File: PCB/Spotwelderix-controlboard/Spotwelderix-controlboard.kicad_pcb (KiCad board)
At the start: 2 copper layers, 65.6 x 60 mm, 35 parts, among them J1 ChargerPower, J2 LEDs, J3 ExtPwr_FAn, P1 Display, P2 PowerPCB, Q1 AO3400A, Q2 AO3400A, Q5 AO3400A, U1 NodeMCU32, U3 LM7805M_TO263

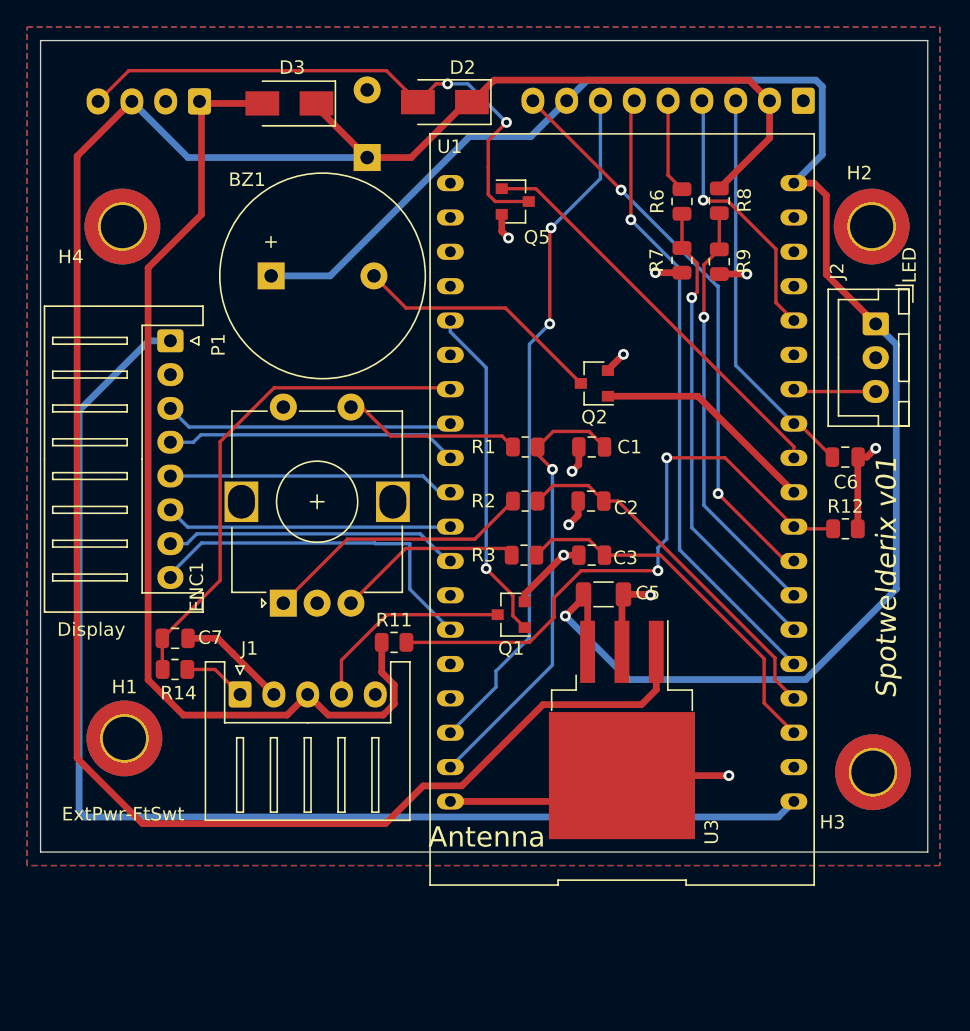
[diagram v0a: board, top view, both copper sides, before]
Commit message: V2 tweaks and tricks
Voltmeasure enable
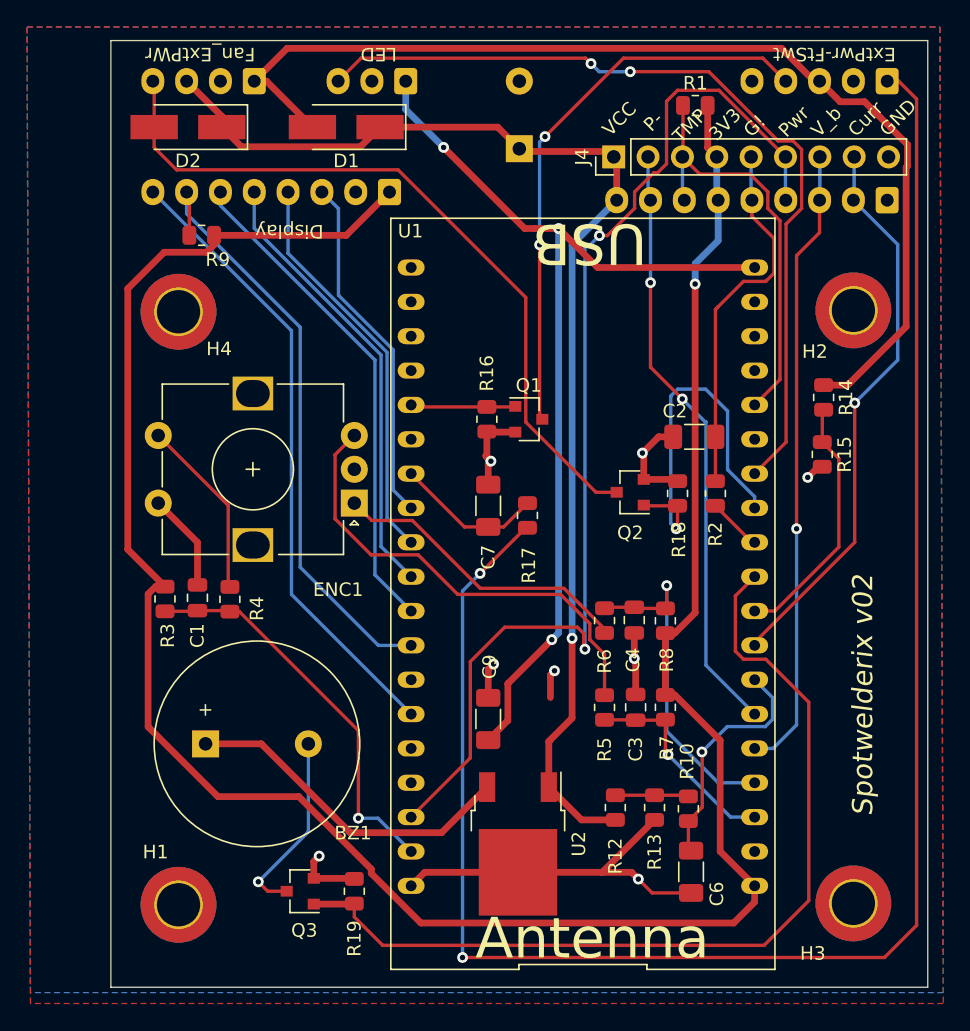
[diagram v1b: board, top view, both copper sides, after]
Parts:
- removed the R6 at (67.4, 31.9)
- added C6: 470p, Capacitor_SMD:C_1206_3216Metric_Pad1.33x1.80mm_HandSolder, F.Cu at (68.1, 81.5)
- added J4: Testpin, Connector_PinHeader_2.54mm:PinHeader_1x09_P2.54mm_Vertical, F.Cu at (62.4, 28.6)
- added R1: 2.5k, Resistor_SMD:R_0805_2012Metric, F.Cu at (68.4, 24.8)
- added R10: 47k, Resistor_SMD:R_0805_2012Metric, F.Cu at (67.9, 76.8)
- added R16: 10k, Resistor_SMD:R_0805_2012Metric, F.Cu at (53.0, 48.0)
- added R18: 10k, Resistor_SMD:R_0805_2012Metric, F.Cu at (67.1, 53.5)
- added R19: 10k, Resistor_SMD:R_0805_2012Metric, F.Cu at (43.2, 82.9)
- added R2: 100, Resistor_SMD:R_0805_2012Metric, F.Cu at (69.9, 53.5)
- added R3: 2.5k, Resistor_SMD:R_0805_2012Metric, F.Cu at (29.2, 61.3)
- added R8: 2.5k, Resistor_SMD:R_0805_2012Metric, F.Cu at (66.2, 62.9)
- added R9: 2.5k, Resistor_SMD:R_0805_2012Metric, F.Cu at (31.9, 34.4)
- C2: renamed from C6; footprint Capacitor_SMD:C_0805_2012Metric -> Capacitor_SMD:C_1206_3216Metric_Pad1.33x1.80mm_HandSolder
- C7: footprint Capacitor_SMD:C_0805_2012Metric -> Capacitor_SMD:C_1206_3216Metric_Pad1.33x1.80mm_HandSolder
- C9: renamed from C5; footprint Capacitor_SMD:C_1206_3216Metric -> Capacitor_SMD:C_1206_3216Metric_Pad1.33x1.80mm_HandSolder
- D1: renamed from D3; footprint Diode_SMD:D_SMA -> Diode_SMD:D_SMA_Handsoldering
- D2: footprint Diode_SMD:D_SMA -> Diode_SMD:D_SMA_Handsoldering
- J1: renamed from J2; moved to B.Cu
- J2: renamed from J1; footprint Connector_JST:JST_XH_S5B-XH-A_1x05_P2.50mm_Horizontal -> Connector_JST:JST_XH_B5B-XH-A_1x05_P2.50mm_Vertical; moved to B.Cu
- P1: footprint Connector_JST:JST_XH_S8B-XH-A_1x08_P2.50mm_Horizontal -> Connector_JST:JST_XH_B8B-XH-A_1x08_P2.50mm_Vertical; moved to B.Cu
- P2: value PowerPCB -> CONN_01X08
- R12: renamed from R8; value 33k -> 15k
- R13: renamed from R9; value 10k -> 2.5k
- R14: renamed from R11; value 33k -> 15k
- R15: renamed from R12; value 10k -> 2.5k
- R7: value 10k -> 2.5k
- U2: renamed from U3; footprint Package_TO_SOT_SMD:TO-263-3_TabPin2 -> Package_TO_SOT_SMD:TO-252-2
- moved J2 65.9 mm to (82.6, 23.0), turned to 180 degrees
- moved R12 45.5 mm to (62.5, 76.7), turned to 90 degrees
- moved Q3 43.4 mm to (39.2, 82.9)
- moved R13 40.6 mm to (65.4, 76.7)
- moved J1 39.1 mm to (47.0, 23.0), turned to 180 degrees
- moved R14 36.6 mm to (77.9, 46.4), turned to 270 degrees
- moved BZ1 34.9 mm to (32.2, 72.0)
- moved R7 33.1 mm to (66.2, 69.3), turned to 90 degrees
- moved C1 31.2 mm to (31.6, 61.2), turned to 90 degrees
- moved R17 28.4 mm to (56.0, 55.1), turned to 270 degrees
- moved C7 25.1 mm to (53.1, 54.4), turned to 90 degrees
- moved R4 24.6 mm to (34.0, 61.3), turned to 90 degrees
- moved Q2 23.1 mm to (63.6, 53.4), turned to 180 degrees
- moved P1 19.6 mm to (45.8, 31.2), turned to 180 degrees
- moved D2 19.1 mm to (30.9, 26.4)
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- renumbered C2 to C4, C4 to C8, Q5 to Q2, Q2 to Q3, R14 to R17, R1 to R4, R3 to R5, R2 to R6
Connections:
- P2 pad 2: VCC -> Shuntvoltage
- P2 pad 3: Gate_logic -> Vbat_ADC
- P2 pad 4: Dallas -> EnableSupply
- P2 pad 5: Probe -> Gate_logic
- P2 pad 6: Vbat_ADC -> +3V3
- P2 pad 7: EnableSupply -> Dallas
- P2 pad 8: +5V -> ProbeADC
- P2 pad 9: Shuntvoltage -> VCC
- R12 pad 2: VCC_ADC -> Net-(R10-Pad2)
- R13 pad 1: VCC_ADC -> Net-(R10-Pad2)
- R7 pad 1: ProbeADC -> UI_RotEnc_B
- R7 pad 2: GND -> +3V3
- U1 pad 11: FAN -> Net-(R2-Pad2)
- U1 pad 12: Gate_logic -> FAN
- U1 pad 18: GND -> Net-(U1-Pad18)
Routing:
- net Net-(J2-Pad1): track 5.30 -> 132.2 mm, vias 0 -> 2
- net +3V3: track 92.0 -> 173.3 mm, vias 0 -> 1
- net VCC: track 167.8 -> 90.4 mm, vias 0 -> 1
- net LED: track 6.12 -> 63.2 mm, vias 0 -> 2
- net BUZZ: track 16.7 -> 67.6 mm
- net EnableSupply: track 51.3 -> 82.2 mm
- net +5V: track 124.7 -> 97.7 mm, vias 1 -> 3
- net Net-(J2-Pad4): track 15.5 -> 42.1 mm, vias 0 -> 2
- net FootSwitch: track 37.4 -> 11.0 mm
- net ExtPWRADC: track 44.7 -> 18.9 mm, vias 2 -> 0
- net Net-(P1-Pad7): track 21.8 -> 45.1 mm
- net Net-(ENC1-PadB): track 13.8 -> 34.5 mm
- net Net-(P1-Pad8): track 26.5 -> 46.5 mm
- net ChargerEna: track 25.0 -> 7.78 mm, vias 1 -> 0
- net Net-(P1-Pad6): track 21.2 -> 36.8 mm
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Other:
- board size 65.6 x 60 mm -> 60.4 x 70 mm
- board text added: "3V3"
- board text added: "Curr"
- board text added: "Fan_ExtPWr"
- board text added: "G!"
- board text added: "GND"
- board text added: "P-"
- board text added: "Pwr"
- board text added: "Spotwelderix v02"
- board text added: "TMP"
- board text added: "USB"
- board text added: "VCC"
- board text added: "V_b"
- board text removed: "Spotwelderix v01"
